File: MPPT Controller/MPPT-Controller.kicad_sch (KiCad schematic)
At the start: 60 parts, among them J1 Conn_01x02_Pin, J2 Conn_01x02_Pin, J3 Conn_01x02_Pin, J4 Conn_01x02_Pin, J6 Conn_01x02_Pin, J7 Conn_01x02_Pin, J8 Conn_01x02_Pin, M1 Fan_4pin, Q1 IRL540N, SW1 SW_SPDT, U1 ADS1115IDGS, U4 LM1117DT-3.3, U5 LM2596S-ADJ, U6 TC4422, U7 ADS1115IDGS

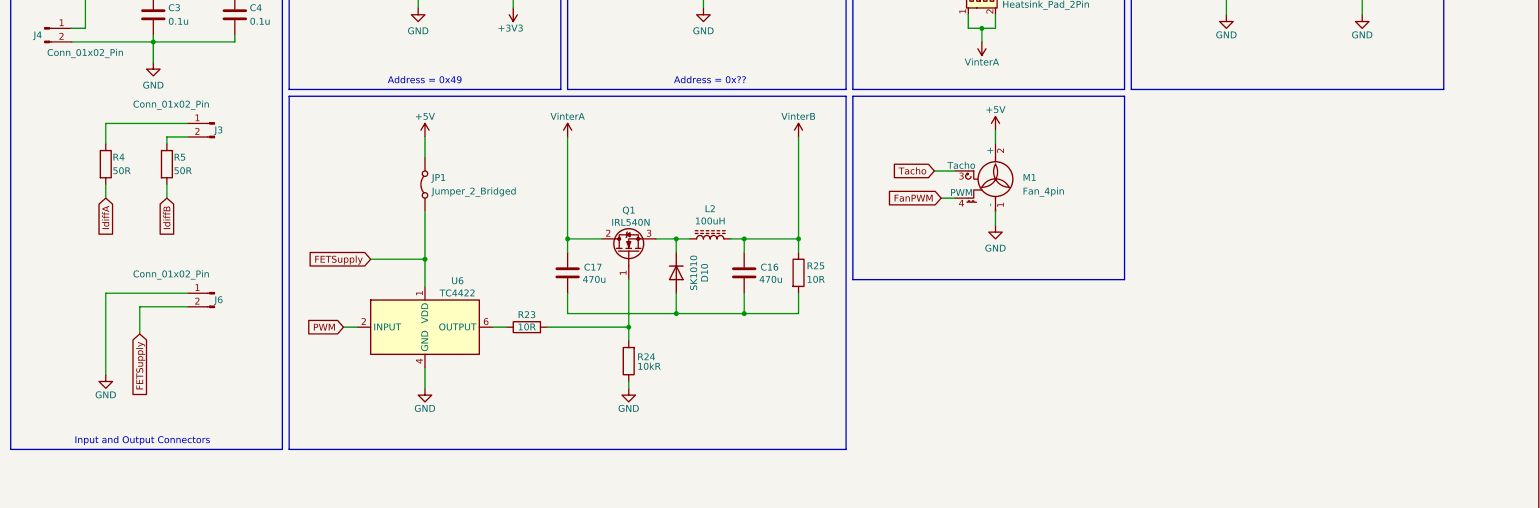
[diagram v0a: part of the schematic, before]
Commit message: usb c
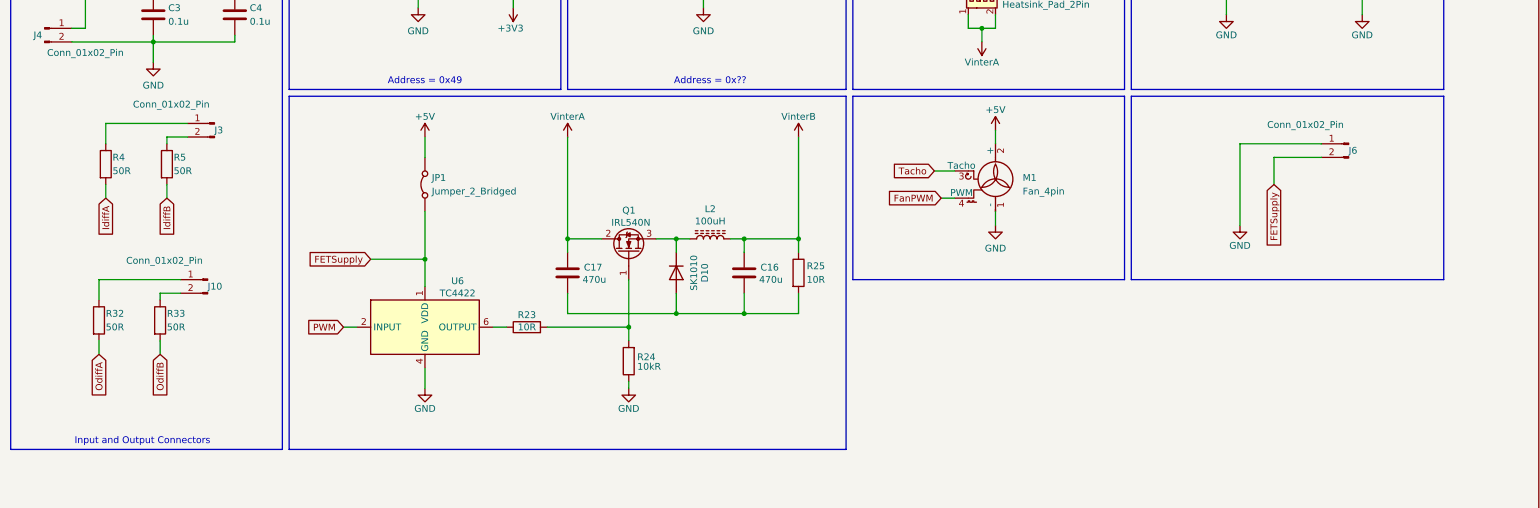
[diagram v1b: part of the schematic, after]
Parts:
- added J10: Conn_01x02_Pin, TerminalBlock:TerminalBlock_Altech_AK300-2_P5.00mm, symbol Connector:Conn_01x02_Pin
- added R32, R33: 50R, Resistor_SMD:R_0603_1608Metric_Pad0.98x0.95mm_HandSolder, symbol Device:R
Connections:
- net OdiffA: now also R32.2
- net OdiffB: now also R33.2
- new net: J10.1 (Pin_1), R32.1
- new net: J10.2 (Pin_2), R33.1
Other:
- moved on the sheet: J6
